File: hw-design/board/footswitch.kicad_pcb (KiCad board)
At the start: 2 copper layers, 249.4 x 58.5 mm, 105 parts, among them J1 CC_MAIN, J2 CC_NEXT, P1 FOOT, P10 CPU_RESET, P2 FOOT, P3 CHAIN, P4 FOOT, P5 FOOT, P6 CONN_01X12, P7 USB_OTG, P8 CONN_01X12, P9 SWD, Q1 2N7002, Q2 BC857, Q3 2N7002, Q4 2N7002, Q5 FDN306P, Q6 IRFML8244TRPBF, Q7 2N7002, Q8 2N7002, U1 ISL83491, U2 NCP1117DT50G, U3 LPC11U24FBD48/401, U4 NCP1117DT33G, Y1 12MHz

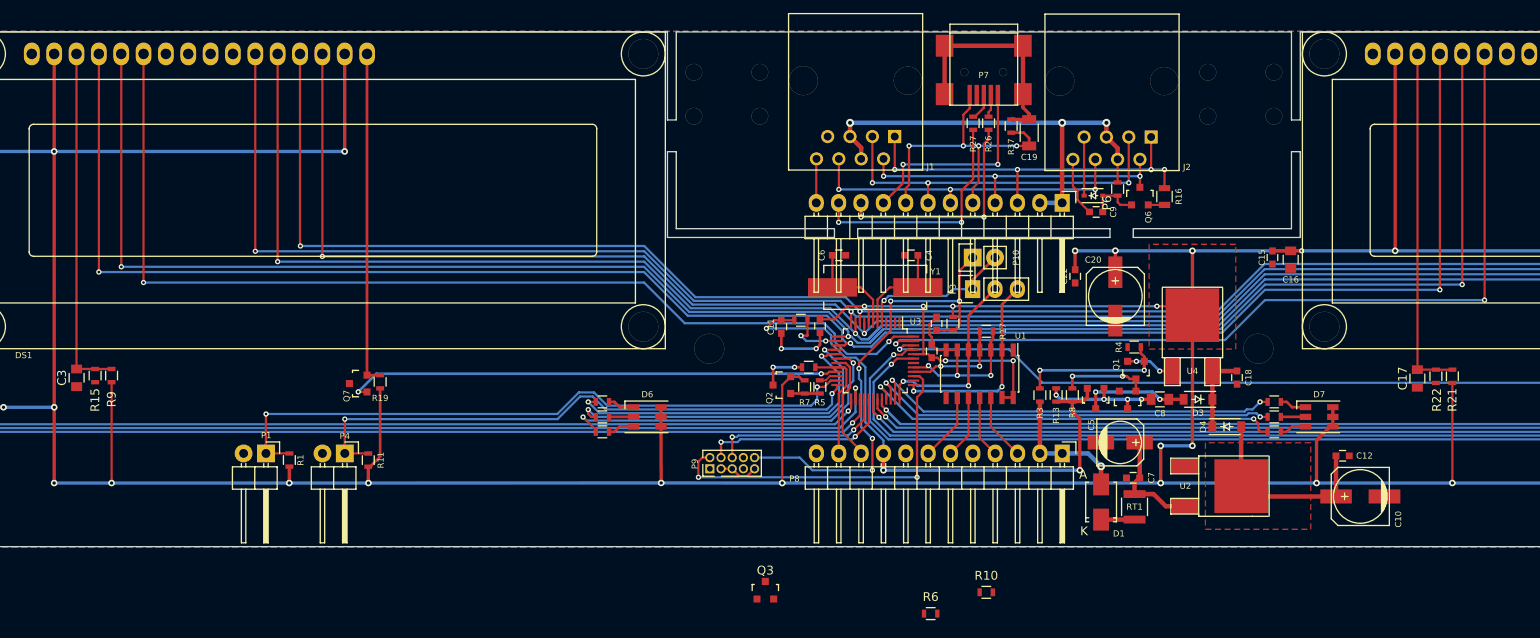
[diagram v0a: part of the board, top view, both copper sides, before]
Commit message: update layout adding last sch changes
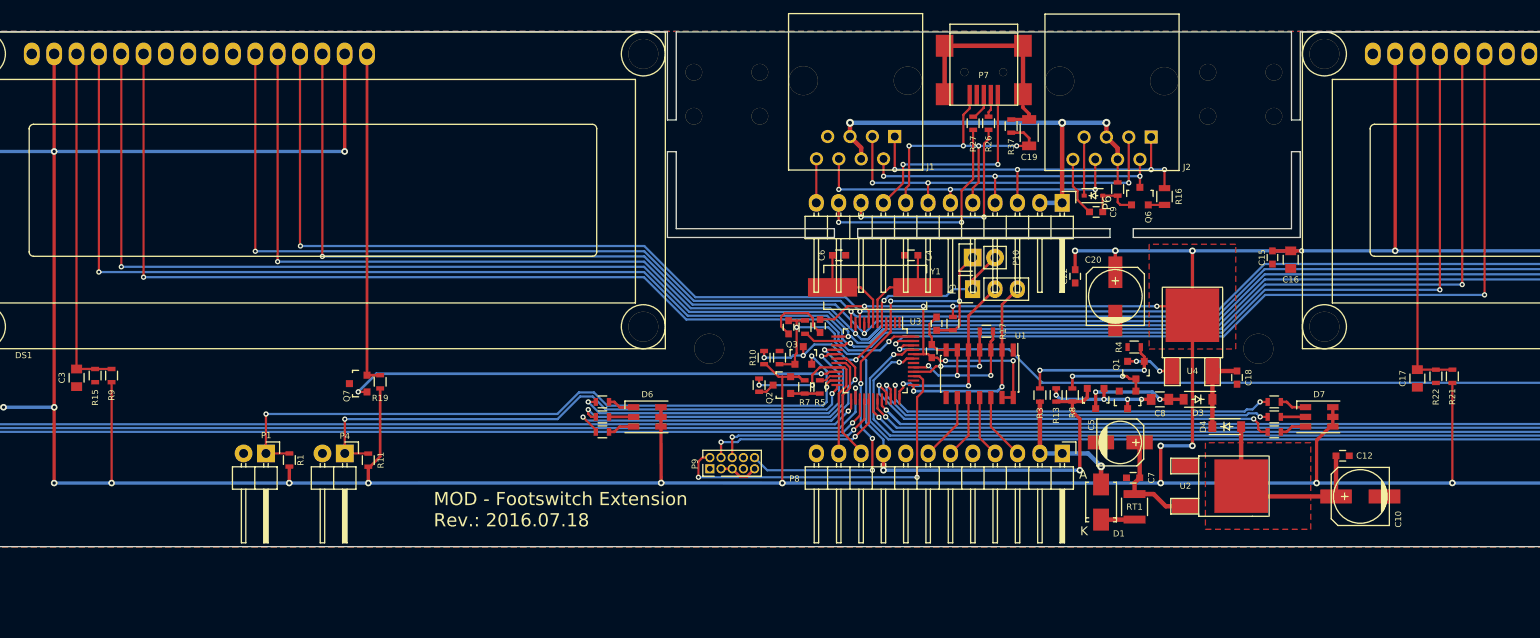
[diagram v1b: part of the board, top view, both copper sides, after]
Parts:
- R6: value 10K -> 100K
- moved R10 36.7 mm to (123.4, 94.0), turned to 270 degrees
- moved R6 33.8 mm to (125.2, 94.0), turned to 270 degrees
- moved Q3 27.0 mm to (127.9, 93.8)
- moved R14 5.99 mm to (122.9, 97.2), turned to 270 degrees
- moved R20 0.92 mm to (128.1, 90.6), turned to 90 degrees
- moved C11 0.82 mm to (126.2, 90.6)
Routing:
- net ISP_TRIGGER: track 0.00 -> 19.2 mm, vias 0 -> 3
- net USB_DP_CPU: track 13.3 -> 21.9 mm, vias 0 -> 2
- net FS1: track 75.7 -> 81.2 mm, vias 2 -> 3
- net Net-(Q2-Pad3): track 5.32 -> 1.92 mm, vias 2 -> 0
- net +3V3: track 651.1 -> 654.3 mm
- net USB_VBUS: track 6.85 -> 3.97 mm, vias 2 -> 0
- net USB_VCC: track 65.0 -> 67.0 mm
- net LED_G3: track 48.2 -> 49.2 mm
- net LCD1_EN: track 118.2 -> 117.5 mm
- net GNDD: track 109.9 -> 110.4 mm, vias 12 -> 10
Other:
- board text added: "MOD - Footswitch Extension Rev.: 2016.07.18"
